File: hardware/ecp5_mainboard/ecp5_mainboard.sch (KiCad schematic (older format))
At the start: 0 parts

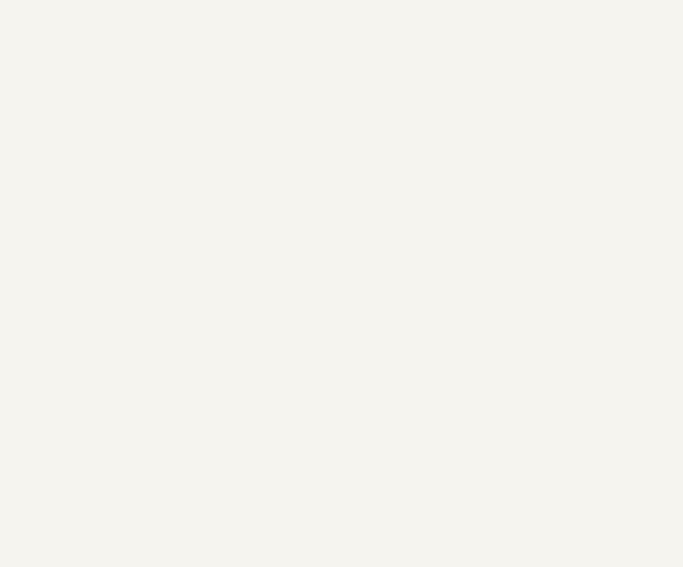
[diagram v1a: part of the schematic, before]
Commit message: hardware/mainboard: Add more mounting holes
Signed-off-by: David Shah <dave@ds0.me>
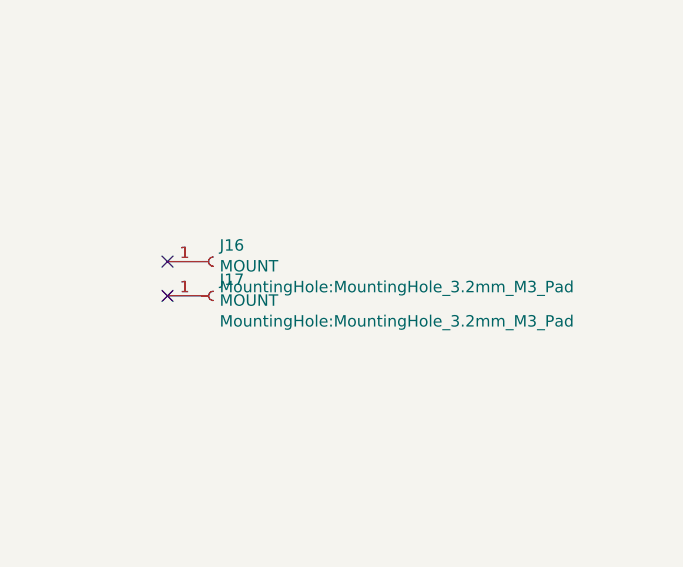
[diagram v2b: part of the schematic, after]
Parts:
- added J16, J17: MOUNT, MountingHole:MountingHole_3.2mm_M3_Pad, symbol Connector:Conn_01x01_Female
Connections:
- no-connect marks 0 -> 2
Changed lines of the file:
@@
 F1 "fpga_io.sch" 50
 $EndSheet
+$Comp
+L Connector:Conn_01x01_Female J16
+U 1 1 5CDA154A
+P 9450 3100
+F 0 "J16" H 9478 3171 50  0000 L CNN
+F 1 "MOUNT" H 9478 3080 50  0000 L CNN
+F 2 "MountingHole:MountingHole_3.2mm_M3_Pad" H 9478 2989 50  0000 L CNN
+F 3 "~" H 9450 3100 50  0001 C CNN
+	1    9450 3100
+	1    0    0    -1
+$EndComp
+$Comp
+L Connector:Conn_01x01_Female J17
+U 1 1 5CDA17E7
+P 9450 3250
+F 0 "J17" H 9478 3321 50  0000 L CNN
+F 1 "MOUNT" H 9478 3230 50  0000 L CNN
+F 2 "MountingHole:MountingHole_3.2mm_M3_Pad" H 9478 3139 50  0000 L CNN
+F 3 "~" H 9450 3250 50  0001 C CNN
+	1    9450 3250
+	1    0    0    -1
+$EndComp
+NoConn ~ 9250 3250
+NoConn ~ 9250 3100
 $EndSCHEMATC
